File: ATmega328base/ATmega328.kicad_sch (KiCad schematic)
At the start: 14 parts, among them J1 Power in, J2 FTDI, U1 AMS1117-5.0, U2 ATmega328P-PU, Y1 16MHz

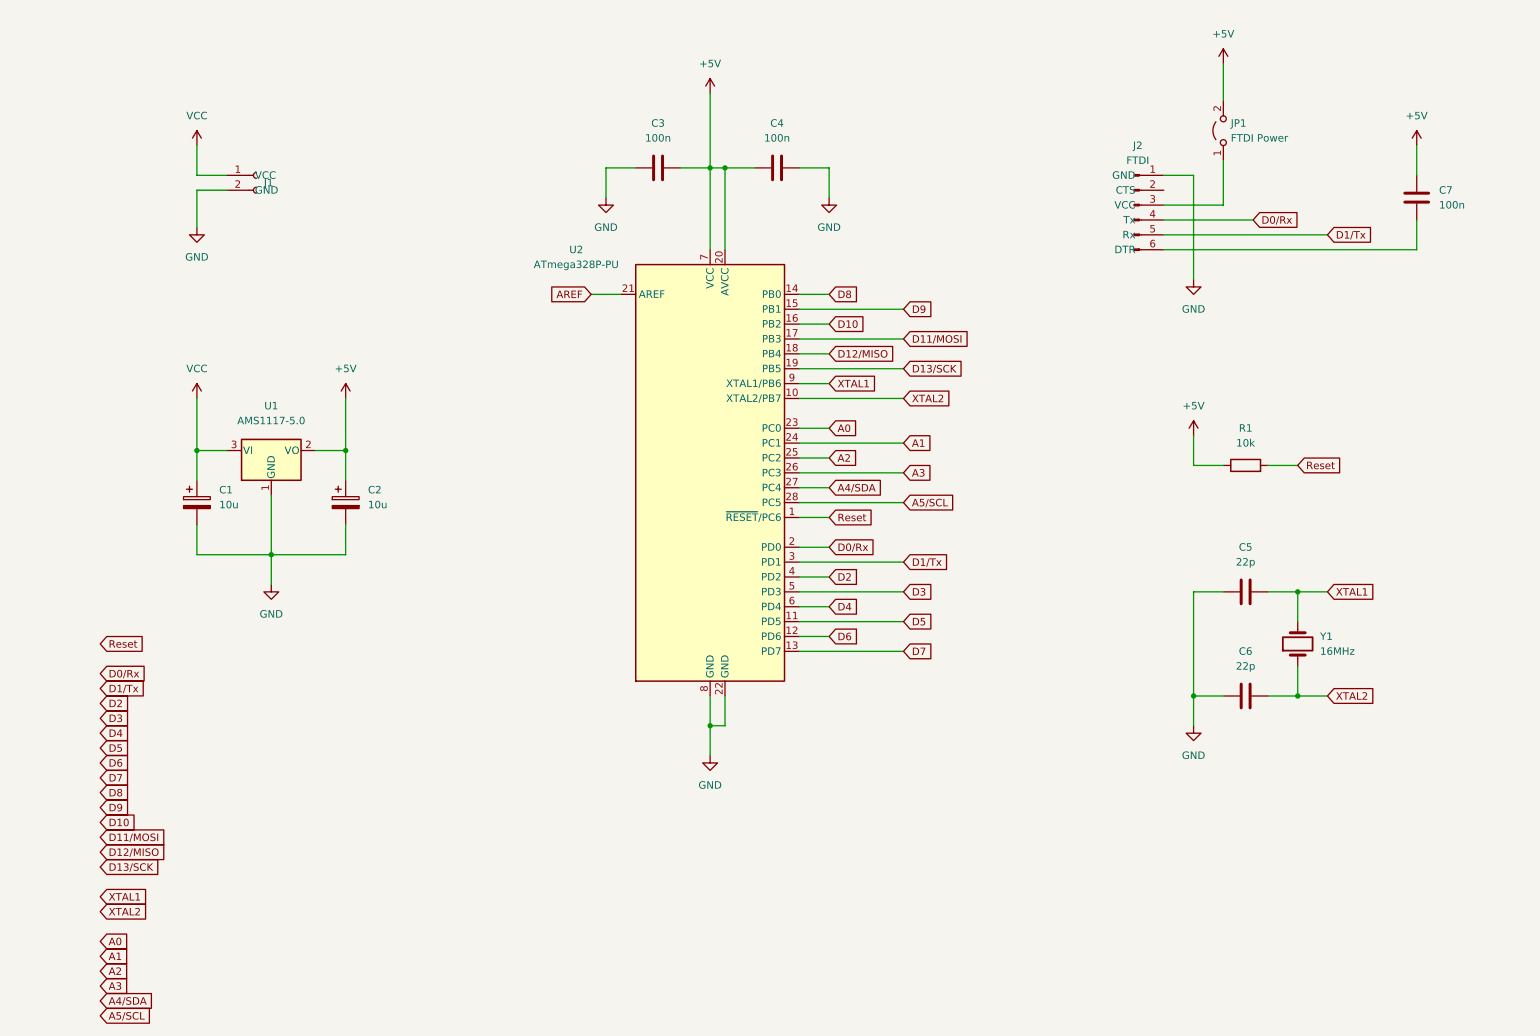
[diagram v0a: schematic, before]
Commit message: atmega base
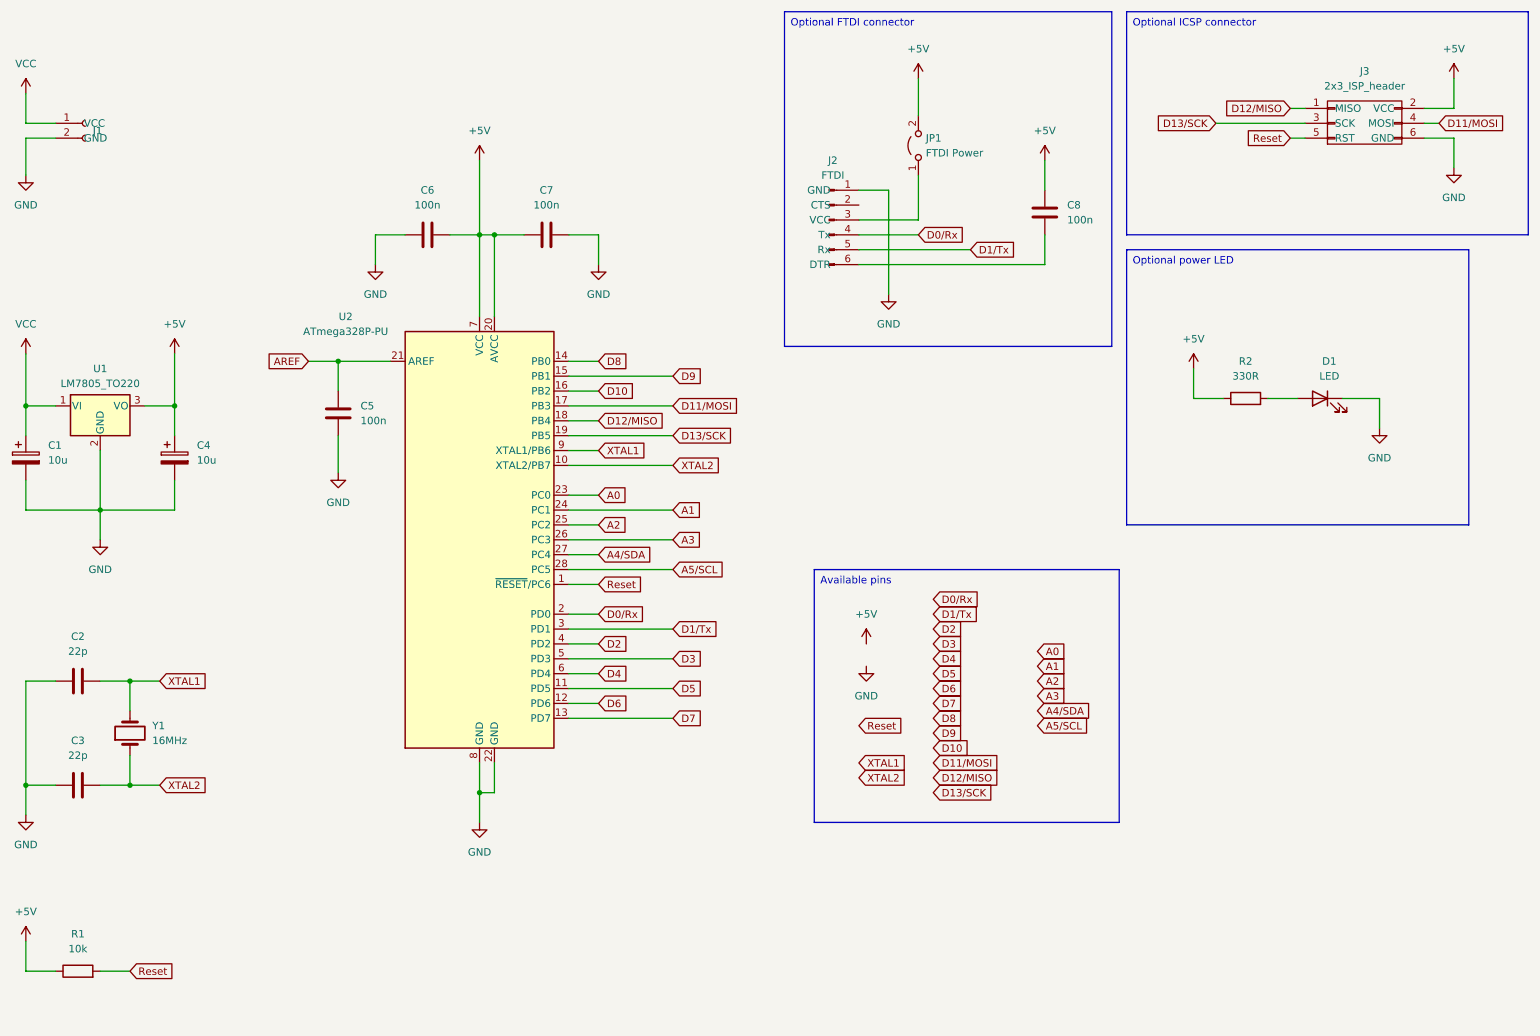
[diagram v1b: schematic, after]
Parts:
- removed C2: 10u, My_Misc:CP_Radial_D5.0mm_P2.00mm_larger, symbol Device:C_Polarized
- removed C4: 100n, My_Misc:C_Disc_D4.3mm_W1.9mm_P5.00mm_large, symbol Device:C
- removed U1: AMS1117-5.0, Package_TO_SOT_SMD:SOT-223-3_TabPin2, symbol Regulator_Linear:AMS1117-5.0
- added C2: 22p, My_Misc:C_Disc_D3.0mm_W1.6mm_P2.50mm_larg, symbol Device:C
- added C4: 10u, My_Misc:CP_Radial_D5.0mm_P2.00mm_larger, symbol Device:C_Polarized
- added C8: 100n, My_Misc:C_Disc_D4.3mm_W1.9mm_P5.00mm_large, symbol Device:C
- added D1: LED, My_Misc:LED_D5.0mm_large, symbol Device:LED
- added J3: 2x3_ISP_header, My_Headers:2x3_ISP_header_large, symbol My_Headers:2x3_ISP_header
- added R2: 330R, My_Misc:R_Axial_DIN0207_L6.3mm_D2.5mm_P10.16mm_Horizontal_large, symbol Device:R
- added U1: LM7805_TO220, My_Misc:TO-220-3_Vertical_larger, symbol Regulator_Linear:LM7805_TO220
- C3: value 100n -> 22p; footprint My_Misc:C_Disc_D4.3mm_W1.9mm_P5.00mm_large -> My_Misc:C_Disc_D3.0mm_W1.6mm_P2.50mm_larg
- C5, C6: value 22p -> 100n; footprint My_Misc:C_Disc_D3.0mm_W1.6mm_P2.50mm_larg -> My_Misc:C_Disc_D4.3mm_W1.9mm_P5.00mm_large
- R1: footprint My_Misc:R_Axial_DIN0207_L6.3mm_D2.5mm_P10.16mm_Horizontal_larger_pads -> My_Misc:R_Axial_DIN0207_L6.3mm_D2.5mm_P10.16mm_Horizontal_large
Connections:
- net +5V: now also C6.1, C4.1, C8.2, J3.2 (VCC), R2.1, U1.3 (VO); no longer C3.1
- net AREF: now also C5.1
- net D11/MOSI: now also J3.4 (MOSI)
- net D12/MISO: now also J3.1 (MISO)
- net D13/SCK: now also J3.3 (SCK)
- net GND: now also C3.1, C5.2, C6.2, C7.1, C2.1, C4.2, D1.1 (K), J3.6 (GND), U1.2 (GND); no longer C3.2, C5.1, C6.1
- net Reset: now also J3.5 (RST)
- net VCC: now also U1.1 (VI)
- net XTAL1: now also C2.2; no longer C5.2
- net XTAL2: now also C3.2; no longer C6.2
- net at J2.6 (DTR): now also C8.1; no longer C7.1
- new net: D1.2 (A), R2.2
